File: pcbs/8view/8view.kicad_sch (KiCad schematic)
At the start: 49 parts, among them J1 Conn_01x10_Female, J2 Conn_01x10_Female, J3 Conn_01x06_Female, J4 Conn_01x06_Female, U1 ATtiny828-A, U2 HDSP-A151, U3 HDSP-A151

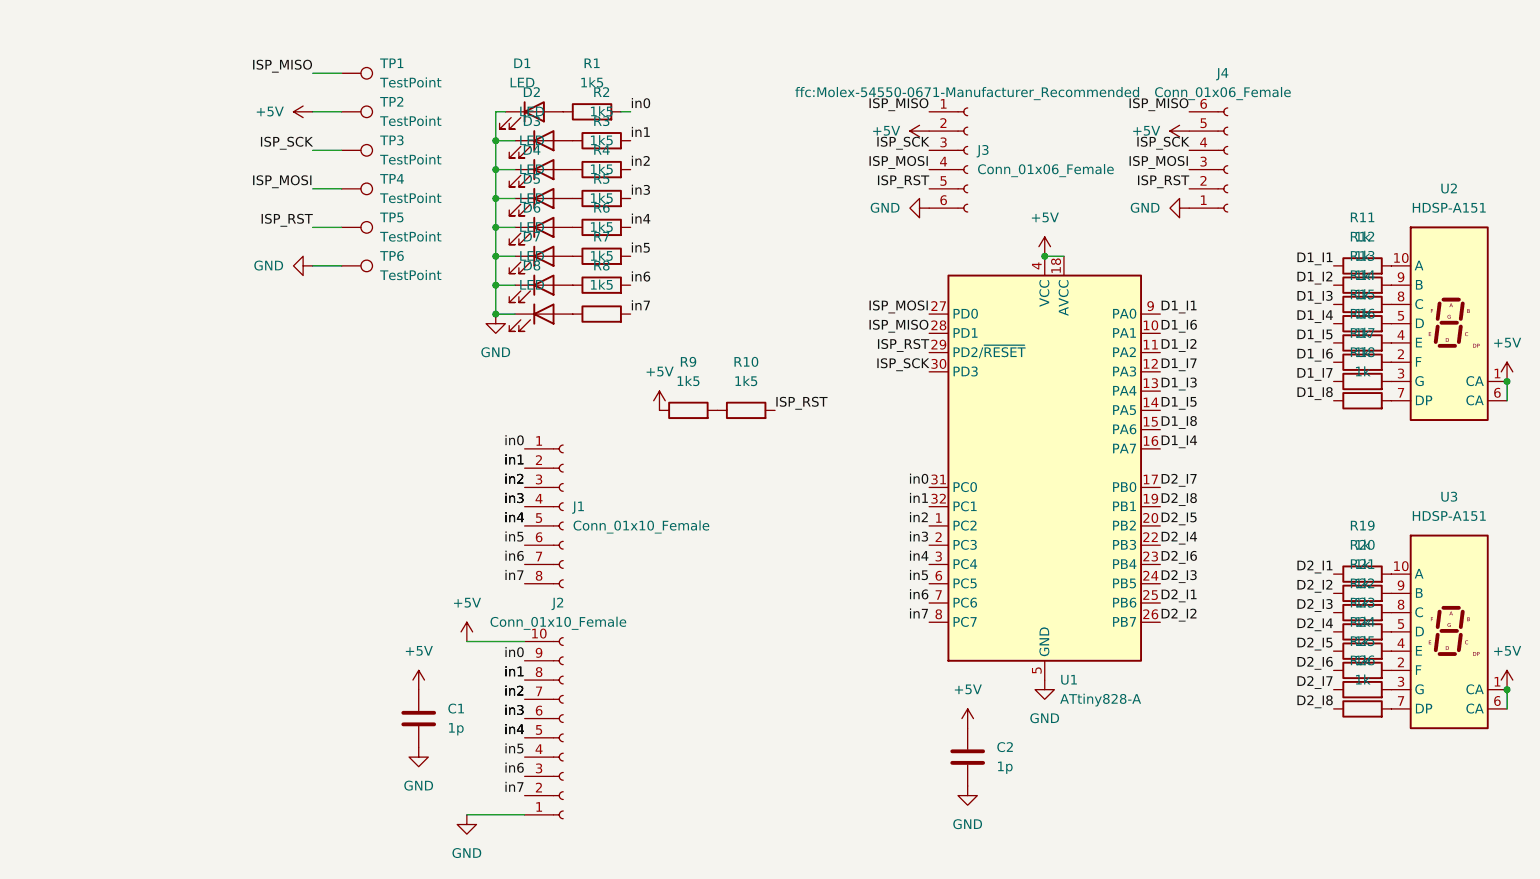
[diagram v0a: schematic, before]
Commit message: 8view: v1.1 touches
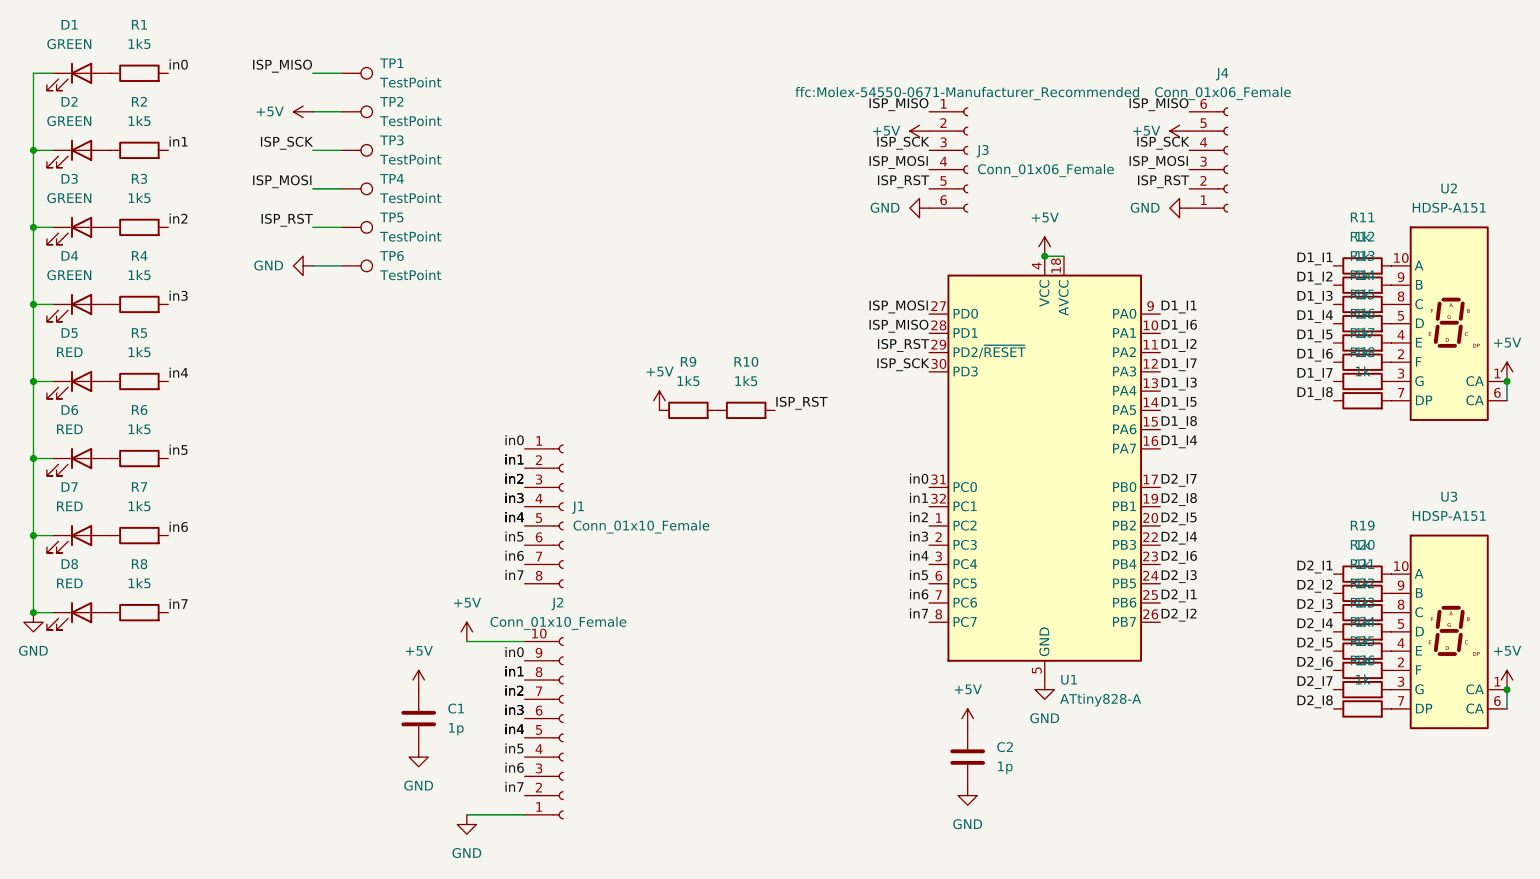
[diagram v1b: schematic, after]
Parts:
- D1, D2, D3, D4: value LED -> GREEN
- D5, D6, D7, D8: value LED -> RED
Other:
- moved on the sheet: D1, D2, D3, D4, D5, D6, D7, D8, R1, R2, R3, R4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
